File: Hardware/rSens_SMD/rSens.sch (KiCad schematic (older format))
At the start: 18 parts, among them U2 MCP6244

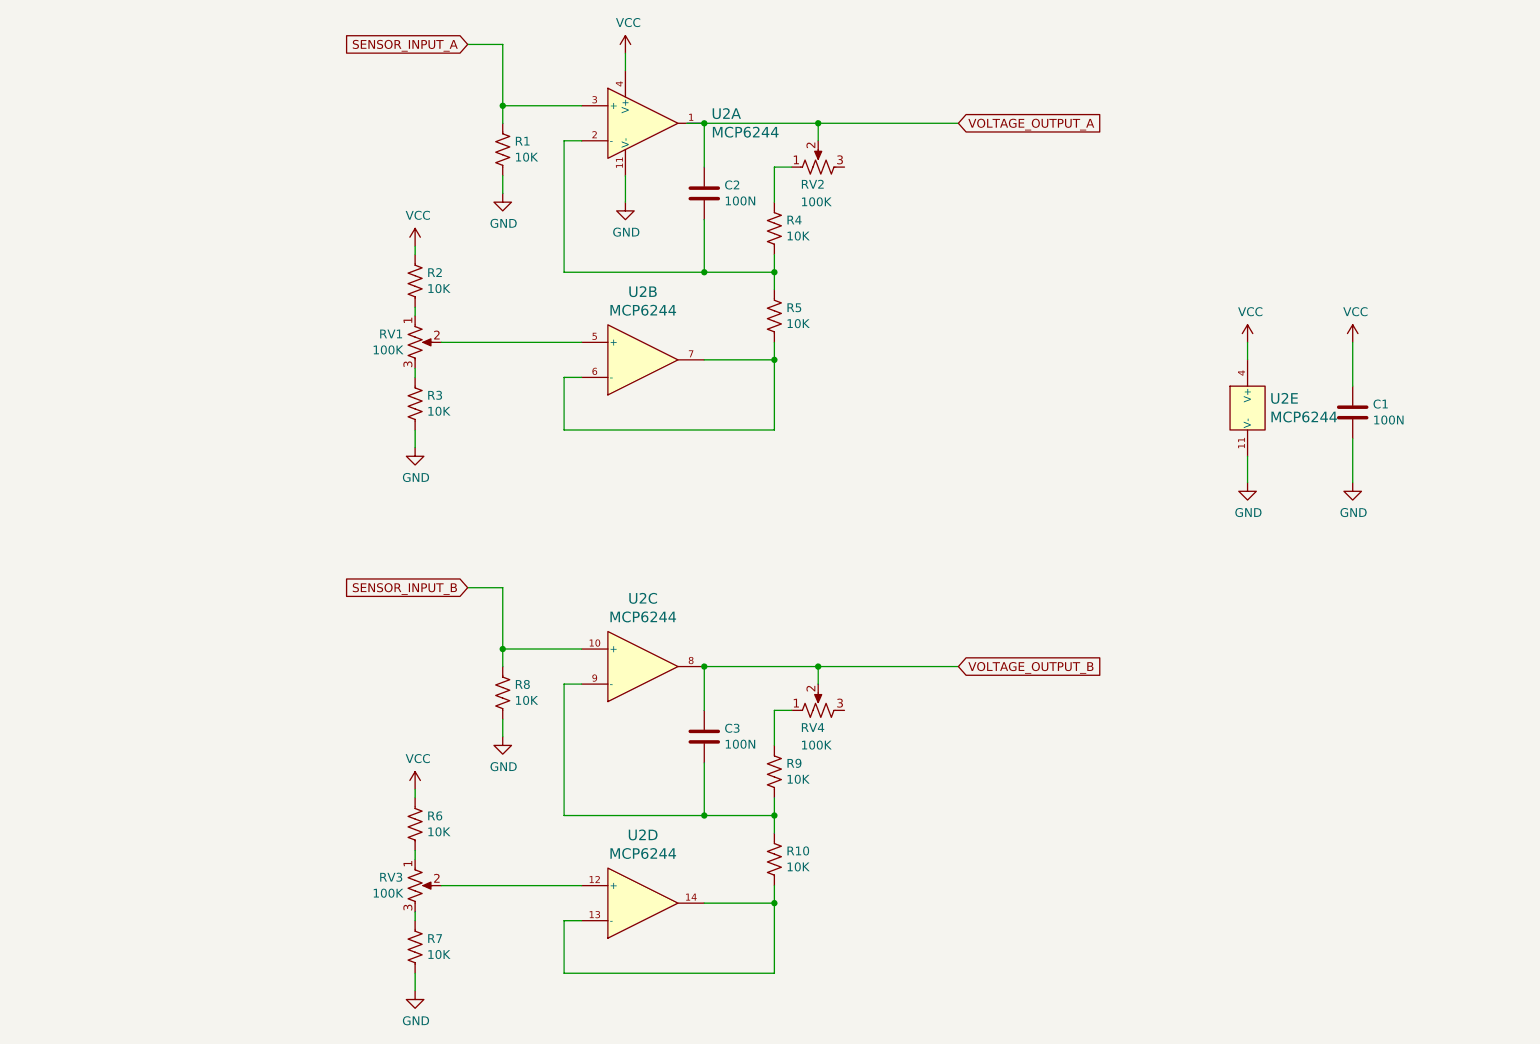
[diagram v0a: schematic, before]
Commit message: Routing in progress
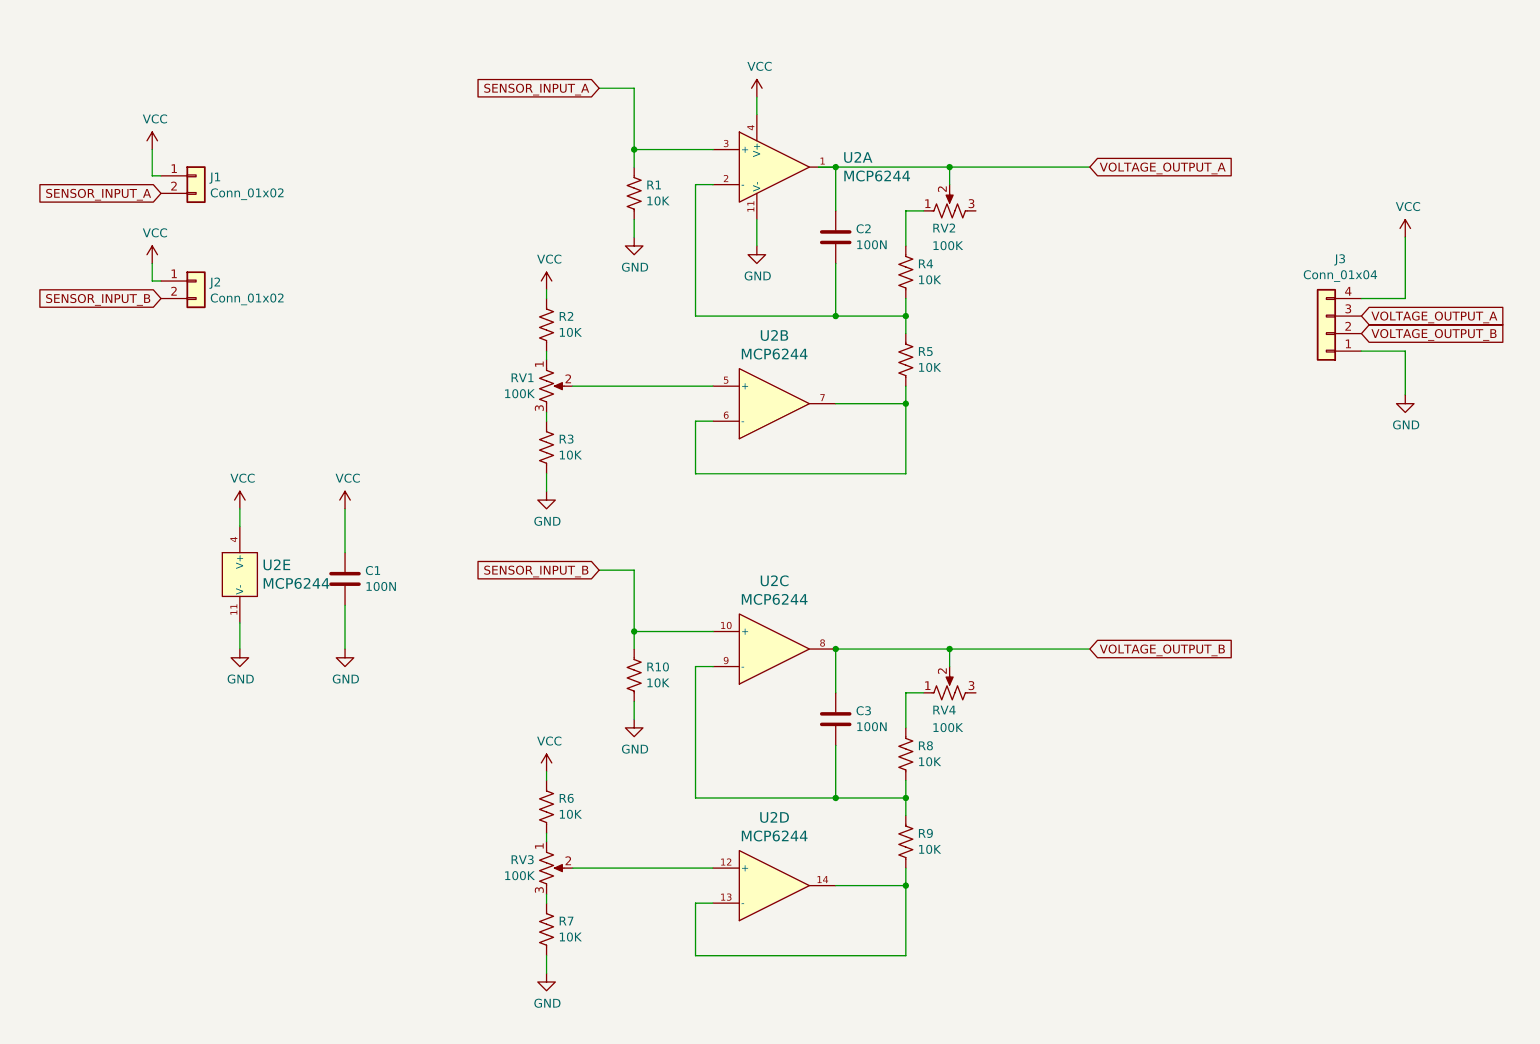
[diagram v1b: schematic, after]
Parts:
- added J1, J2: Conn_01x02, rSens:rSens_Pad_1x02, symbol Connector_Generic:Conn_01x02
- added J3: Conn_01x04, rSens:rSens_Pad_1x04, symbol Connector_Generic:Conn_01x04
- C1, C2, C3: footprint Capacitor_SMD:C_0603_1608Metric -> Capacitor_SMD:C_0805_2012Metric_Pad1.18x1.45mm_HandSolder
- R1: footprint Resistor_SMD:R_0603_1608Metric -> Resistor_THT:R_Axial_DIN0309_L9.0mm_D3.2mm_P12.70mm_Horizontal
- R10: renamed from R8; footprint Resistor_SMD:R_0603_1608Metric -> Resistor_THT:R_Axial_DIN0309_L9.0mm_D3.2mm_P12.70mm_Horizontal
- R2, R3, R4, R5, R6, R7: footprint Resistor_SMD:R_0603_1608Metric -> Resistor_SMD:R_0805_2012Metric_Pad1.20x1.40mm_HandSolder
- R8: renamed from R9; footprint Resistor_SMD:R_0603_1608Metric -> Resistor_SMD:R_0805_2012Metric_Pad1.20x1.40mm_HandSolder
- R9: renamed from R10; footprint Resistor_SMD:R_0603_1608Metric -> Resistor_SMD:R_0805_2012Metric_Pad1.20x1.40mm_HandSolder
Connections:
- net GND: now also J3.1 (Pin_1)
- net SENSOR_INPUT_A: now also J1.2 (Pin_2)
- net SENSOR_INPUT_B: now also J2.2 (Pin_2)
- net VCC: now also J1.1 (Pin_1), J2.1 (Pin_1), J3.4 (Pin_4)
- net VOLTAGE_OUTPUT_A: now also J3.3 (Pin_3)
- net VOLTAGE_OUTPUT_B: now also J3.2 (Pin_2)
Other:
- moved on the sheet: C1, C2, C3, R1, R10, R2, R3, R4, R5, R6, R7, R8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

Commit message: Routing done
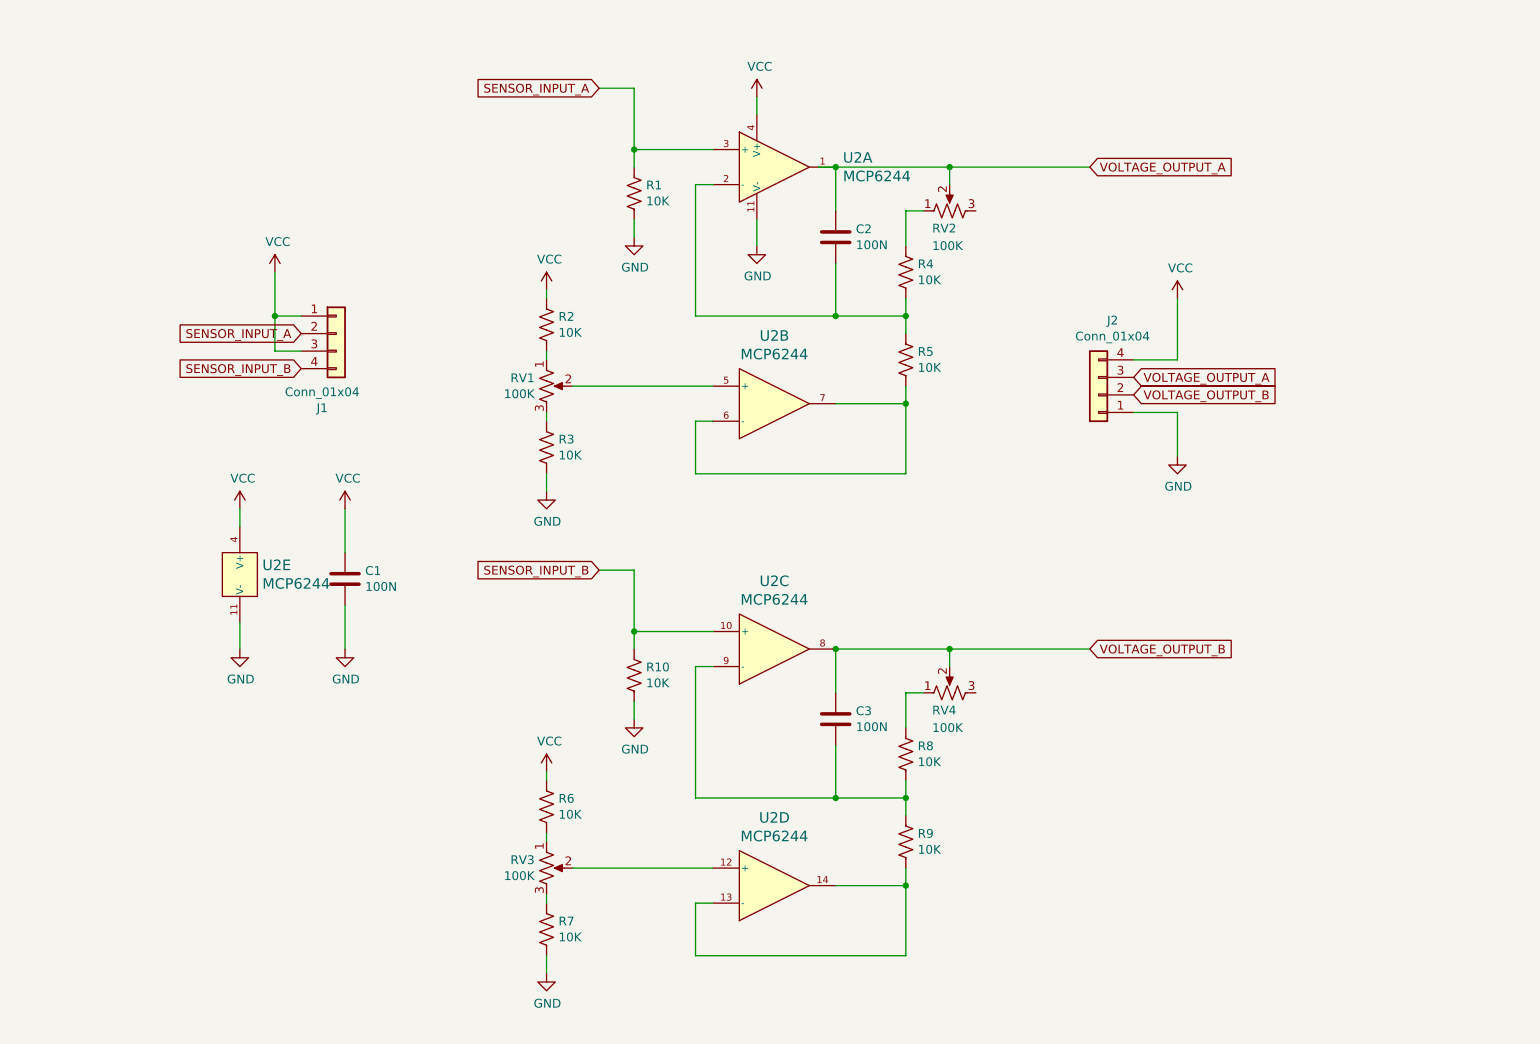
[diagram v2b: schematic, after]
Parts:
- removed J1, J2: Conn_01x02, rSens:rSens_Pad_1x02, symbol Connector_Generic:Conn_01x02
- added J1: Conn_01x04, rSens:rSens_Pad_1x04, symbol Connector_Generic:Conn_01x04
- renumbered J3 to J2
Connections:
- net SENSOR_INPUT_A: now also J1.2 (Pin_2)
- net SENSOR_INPUT_B: now also J1.4 (Pin_4)
- net VCC: now also J1.1 (Pin_1), J1.3 (Pin_3)
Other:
- moved on the sheet: J2
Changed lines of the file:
@@
 EESchema Schematic File Version 4
+LIBS:rSens-cache
 EELAYER 26 0
 EELAYER END
@@
 Wire Wire Line
 	6200 2050 6200 2200
-$Comp
-L Connector_Generic:Conn_01x02 J1
-U 1 1 60302574
-P 3000 1800
-F 0 "J1" H 3080 1792 50  0000 L CNN
-F 1 "Conn_01x02" H 3080 1701 50  0000 L CNN
-F 2 "rSens:rSens_Pad_1x02" H 3000 1800 50  0001 C CNN
-F 3 "~" H 3000 1800 50  0001 C CNN
-	1    3000 1800
-	1    0    0    -1
-$EndComp
-$Comp
-L Connector_Generic:Conn_01x02 J2
-U 1 1 603074C9
-P 3000 2400
-F 0 "J2" H 3080 2392 50  0000 L CNN
-F 1 "Conn_01x02" H 3080 2301 50  0000 L CNN
-F 2 "rSens:rSens_Pad_1x02" H 3000 2400 50  0001 C CNN
-F 3 "~" H 3000 2400 50  0001 C CNN
-	1    3000 2400
-	1    0    0    -1
-$EndComp
-Text GLabel 2800 1900 0    50   Input ~ 0
+Text GLabel 3600 2700 0    50   Input ~ 0
 SENSOR_INPUT_A
-Text GLabel 2800 2500 0    50   Input ~ 0
+Text GLabel 3600 2900 0    50   Input ~ 0
 SENSOR_INPUT_B
 $Comp
 L power:VCC #PWR0113
 U 1 1 6030C527
-P 2750 2300
-F 0 "#PWR0113" H 2750 2150 50  0001 C CNN
-F 1 "VCC" H 2767 2473 50  0000 C CNN
-F 2 "" H 2750 2300 50  0001 C CNN
-F 3 "" H 2750 2300 50  0001 C CNN
-	1    2750 2300
-	1    0    0    -1
-$EndComp
-$Comp
-L power:VCC #PWR0114
-U 1 1 6030EA4D
-P 2750 1650
-F 0 "#PWR0114" H 2750 1500 50  0001 C CNN
-F 1 "VCC" H 2767 1823 50  0000 C CNN
-F 2 "" H 2750 1650 50  0001 C CNN
-F 3 "" H 2750 1650 50  0001 C CNN
-	1    2750 1650
-	1    0    0    -1
-$EndComp
-Wire Wire Line
-	2800 1800 2750 1800
-Wire Wire Line
-	2750 1800 2750 1650
-Wire Wire Line
-	2800 2400 2750 2400
-Wire Wire Line
-	2750 2400 2750 2300
-$Comp
-L Connector_Generic:Conn_01x04 J3
-U 1 1 6036460C
-P 9450 2700
-F 0 "J3" H 9370 2275 50  0000 C CNN
-F 1 "Conn_01x04" H 9370 2366 50  0000 C CNN
-F 2 "rSens:rSens_Pad_1x04" H 9450 2700 50  0001 C CNN
-F 3 "~" H 9450 2700 50  0001 C CNN
-	1    9450 2700
-	-1   0    0    1
-$EndComp
-Text GLabel 9650 2600 2    50   Input ~ 0
+P 3450 2350
+F 0 "#PWR0113" H 3450 2200 50  0001 C CNN
+F 1 "VCC" H 3467 2523 50  0000 C CNN
+F 2 "" H 3450 2350 50  0001 C CNN
+F 3 "" H 3450 2350 50  0001 C CNN
+	1    3450 2350
+	1    0    0    -1
+$EndComp
+Text GLabel 8350 2950 2    50   Input ~ 0
 VOLTAGE_OUTPUT_A
-Text GLabel 9650 2700 2    50   Input ~ 0
+Text GLabel 8350 3050 2    50   Input ~ 0
 VOLTAGE_OUTPUT_B
 $Comp
 L power:VCC #PWR0115
 U 1 1 60364A29
-P 9900 2150
-F 0 "#PWR0115" H 9900 2000 50  0001 C CNN
-F 1 "VCC" H 9917 2323 50  0000 C CNN
-F 2 "" H 9900 2150 50  0001 C CNN
-F 3 "" H 9900 2150 50  0001 C CNN
-	1    9900 2150
+P 8600 2500
+F 0 "#PWR0115" H 8600 2350 50  0001 C CNN
+F 1 "VCC" H 8617 2673 50  0000 C CNN
+F 2 "" H 8600 2500 50  0001 C CNN
+F 3 "" H 8600 2500 50  0001 C CNN
+	1    8600 2500
 	1    0    0    -1
 $EndComp
@@
 L power:GND #PWR0116
 U 1 1 60364B2E
-P 9900 3050
-F 0 "#PWR0116" H 9900 2800 50  0001 C CNN
-F 1 "GND" H 9905 2877 50  0000 C CNN
-F 2 "" H 9900 3050 50  0001 C CNN
-F 3 "" H 9900 3050 50  0001 C CNN
-	1    9900 3050
-	1    0    0    -1
-$EndComp
-Wire Wire Line
-	9900 2150 9900 2500
-Wire Wire Line
-	9900 2500 9650 2500
-Wire Wire Line
-	9650 2800 9900 2800
-Wire Wire Line
-	9900 2800 9900 3050
+P 8600 3400
+F 0 "#PWR0116" H 8600 3150 50  0001 C CNN
+F 1 "GND" H 8605 3227 50  0000 C CNN
+F 2 "" H 8600 3400 50  0001 C CNN
+F 3 "" H 8600 3400 50  0001 C CNN
+	1    8600 3400
+	1    0    0    -1
+$EndComp
+Wire Wire Line
+	8600 2500 8600 2850
+Wire Wire Line
+	8600 2850 8350 2850
+Wire Wire Line
+	8350 3150 8600 3150
+Wire Wire Line
+	8600 3150 8600 3400
+Wire Wire Line
+	3600 2600 3450 2600
+Wire Wire Line
+	3450 2600 3450 2350
+Wire Wire Line
+	3600 2800 3450 2800
+Wire Wire Line
+	3450 2800 3450 2600
+Connection ~ 3450 2600
+$Comp
+L Connector_Generic:Conn_01x04 J2
+U 1 1 6036460C
+P 8150 3050
+F 0 "J2" H 8070 2625 50  0000 C CNN
+F 1 "Conn_01x04" H 8070 2716 50  0000 C CNN
+F 2 "rSens:rSens_Pad_1x04" H 8150 3050 50  0001 C CNN
+F 3 "~" H 8150 3050 50  0001 C CNN
+	1    8150 3050
+	-1   0    0    1
+$EndComp
+$Comp
+L Connector_Generic:Conn_01x04 J1
+U 1 1 6042322A
+P 3800 2700
+F 0 "J1" H 3720 2275 50  0000 C CNN
+F 1 "Conn_01x04" H 3720 2366 50  0000 C CNN
+F 2 "rSens:rSens_Pad_1x04" H 3800 2700 50  0001 C CNN
+F 3 "~" H 3800 2700 50  0001 C CNN
+	1    3800 2700
+	1    0    0    -1
+$EndComp
 $EndSCHEMATC
